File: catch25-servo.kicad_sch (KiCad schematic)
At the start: 1 part

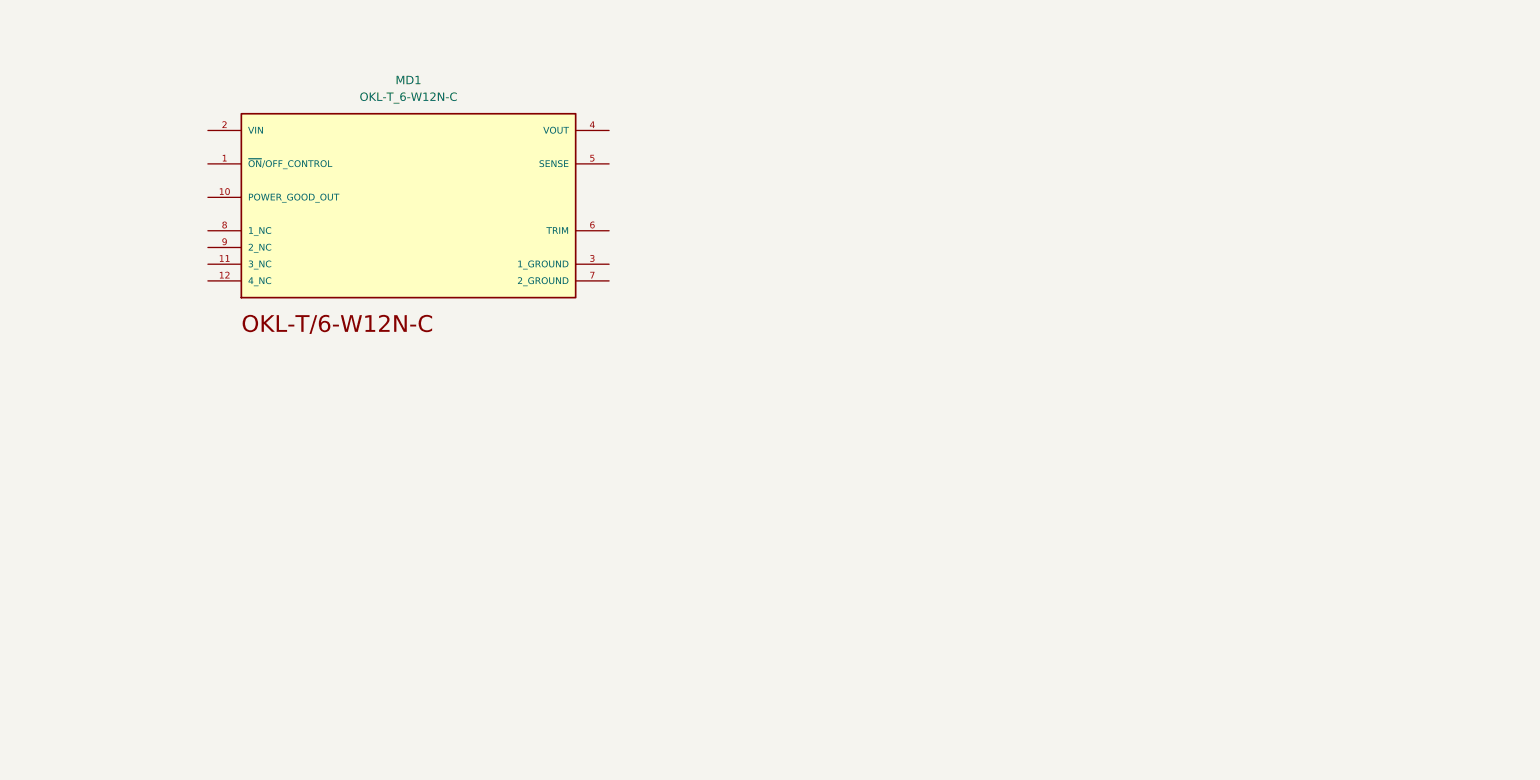
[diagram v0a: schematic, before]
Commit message: update files
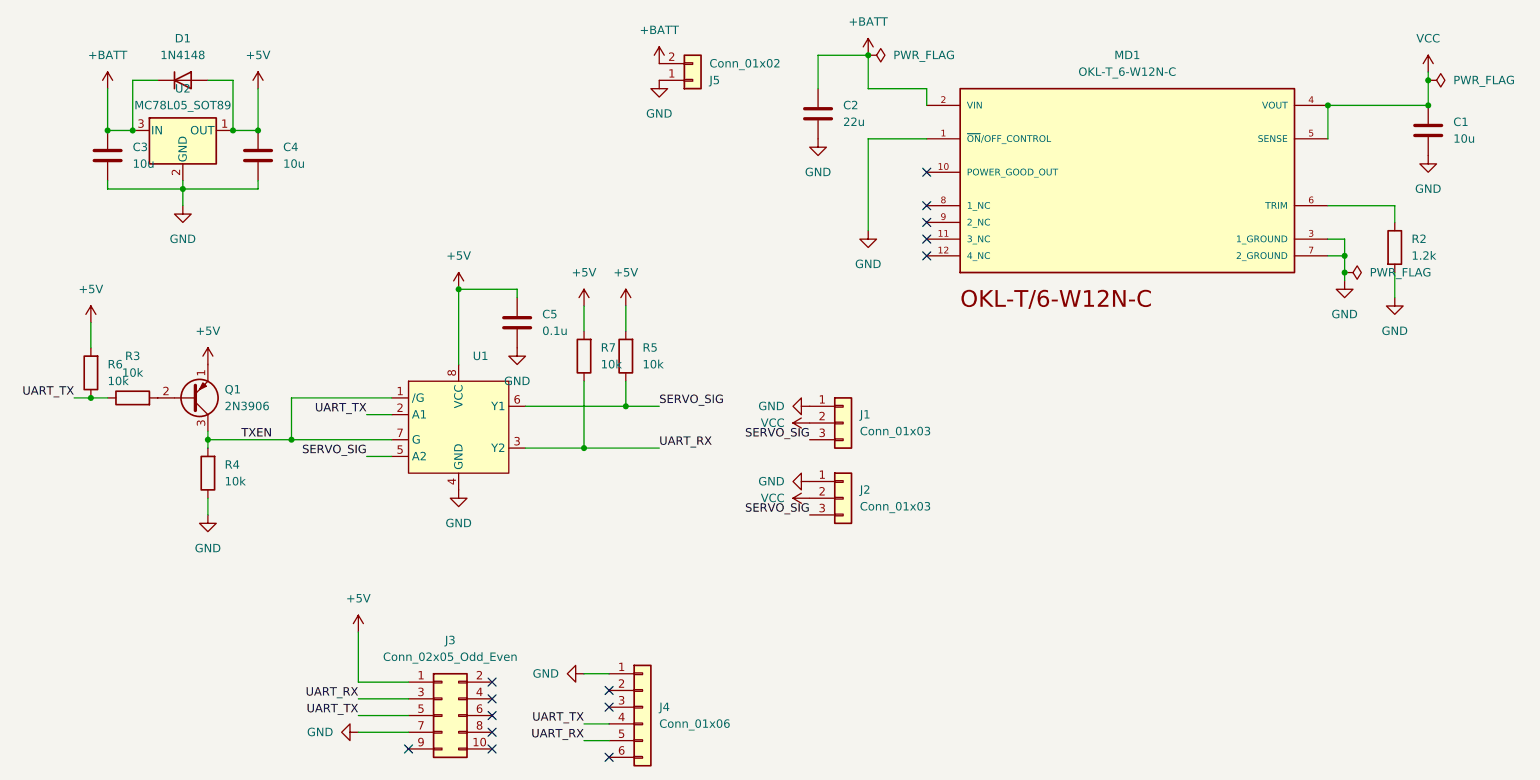
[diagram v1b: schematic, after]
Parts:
- added C1, C3, C4: 10u, Capacitor_SMD:C_0603_1608Metric_Pad1.08x0.95mm_HandSolder, symbol Device:C
- added C2: 22u, Capacitor_SMD:C_0603_1608Metric_Pad1.08x0.95mm_HandSolder, symbol Device:C
- added C5: 0.1u, Capacitor_SMD:C_0603_1608Metric_Pad1.08x0.95mm_HandSolder, symbol Device:C
- added D1: 1N4148, Diode_THT:D_DO-35_SOD27_P7.62mm_Horizontal, symbol Diode:1N4148
- added J1, J2: Conn_01x03, Connector_Molex:Molex_SPOX_5268-03A_1x03_P2.50mm_Horizontal, symbol Connector_Generic:Conn_01x03
- added J3: Conn_02x05_Odd_Even, Connector_PinSocket_2.54mm:PinSocket_2x05_P2.54mm_Horizontal, symbol Connector_Generic:Conn_02x05_Odd_Even
- added J4: Conn_01x06, Connector_PinSocket_2.54mm:PinSocket_1x06_P2.54mm_Vertical, symbol Connector_Generic:Conn_01x06
- added J5: Conn_01x02, Connector_AMASS:AMASS_XT30PW-M_1x02_P2.50mm_Horizontal, symbol Connector_Generic:Conn_01x02
- added Q1: 2N3906, Package_TO_SOT_THT:TO-92_Inline, symbol Transistor_BJT:2N3906
- added R2: 1.2k, Resistor_SMD:R_0603_1608Metric_Pad0.98x0.95mm_HandSolder, symbol Device:R
- added R3, R4, R5, R6, R7: 10k, Resistor_SMD:R_0603_1608Metric_Pad0.98x0.95mm_HandSolder, symbol Device:R
- added U1: ~, Package_SO:VSSOP-8_2.3x2mm_P0.5mm, symbol Library:TC7WH241FK
- added U2: MC78L05_SOT89, Package_TO_SOT_SMD:SOT-89-3, symbol Regulator_Linear:MC78L05_SOT89
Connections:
- net GND: now reaches MD1.1 (~{ON}/OFF_CONTROL)
- net GND: now also MD1.3 (1_GROUND), MD1.7 (2_GROUND), C1.2, C2.2, C3.2, C4.2, C5.2, J1.1 (Pin_1), J2.1 (Pin_1), J3.7 (Pin_7), J4.1 (Pin_1), J5.1 (Pin_1), R2.2, R4.1, U1.4 (GND), U2.2 (GND)
- net +BATT: now reaches MD1.2 (VIN)
- net +BATT: now also C2.1, C3.1, D1.1 (K), J5.2 (Pin_2), U2.3 (IN)
- net VCC: now reaches MD1.4 (VOUT)
- net VCC: now also MD1.5 (SENSE), C1.1, J1.2 (Pin_2), J2.2 (Pin_2)
- net at MD1.6 (TRIM): now also R2.1
- new net: Q1.2 (B), R3.2
- new net +5V: C4.1, C5.1, D1.2 (A), J3.1 (Pin_1), Q1.1 (E), R5.2, R6.2, R7.2, U1.8 (VCC), U2.1 (OUT)
- new net SERVO_SIG: J1.3 (Pin_3), J2.3 (Pin_3), R5.1, U1.5 (A2), U1.6 (Y1)
- new net TXEN: Q1.3 (C), R4.2, U1.1 (/G), U1.7 (G)
- new net UART_RX: J3.3 (Pin_3), J4.5 (Pin_5), R7.1, U1.3 (Y2)
- new net UART_TX: J3.5 (Pin_5), J4.4 (Pin_4), R3.1, R6.1, U1.2 (A1)
- no-connect marks 0 -> 14
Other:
- moved on the sheet: MD1
